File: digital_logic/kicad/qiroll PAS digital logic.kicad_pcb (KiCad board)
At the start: 2 copper layers, 53.3 x 45.7 mm, 43 parts, among them J1 led_sw1, J2 mode_thr_batt, J3 pas_sense, J4 brk_sense, J5 jumper, U1 14538, U2 4023, U3 4027, U4 14538, U5 L7805, U6 4081, U7 4047, U8 74VHC1G32

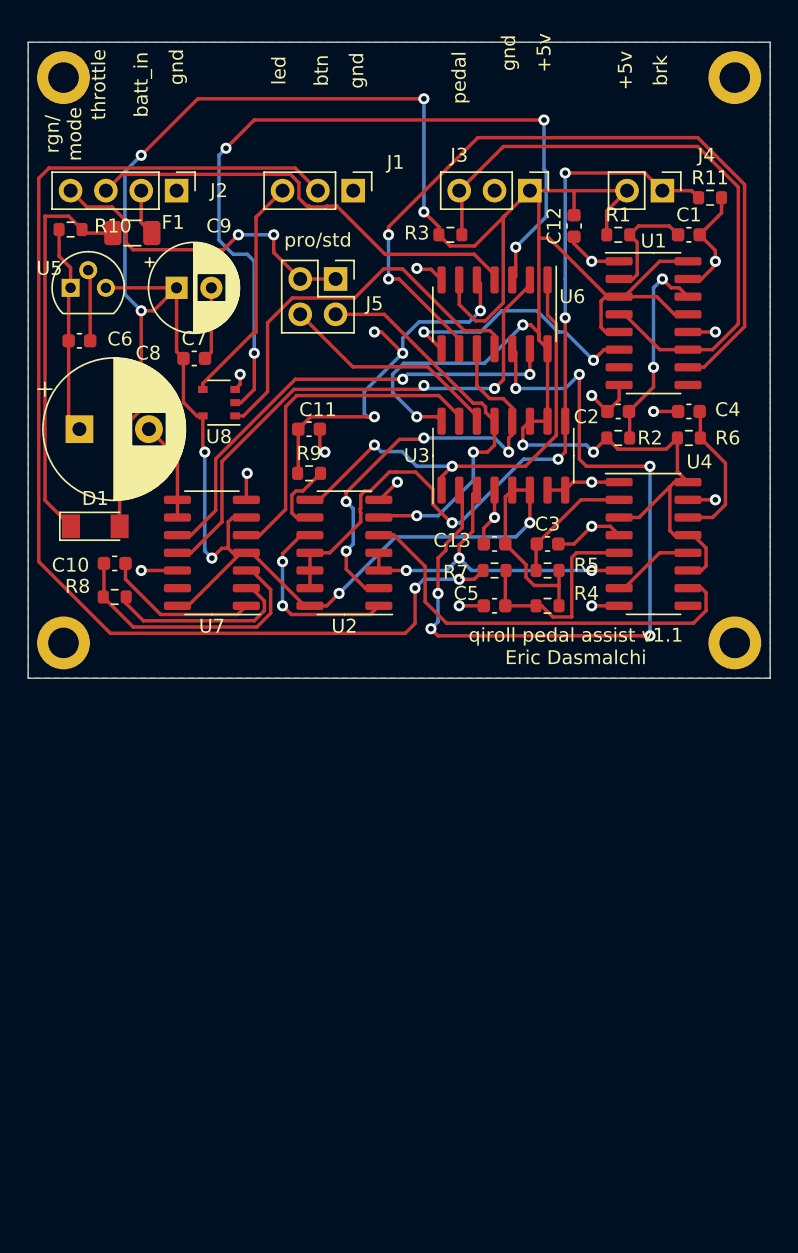
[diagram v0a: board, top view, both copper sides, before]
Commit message: trial component placement
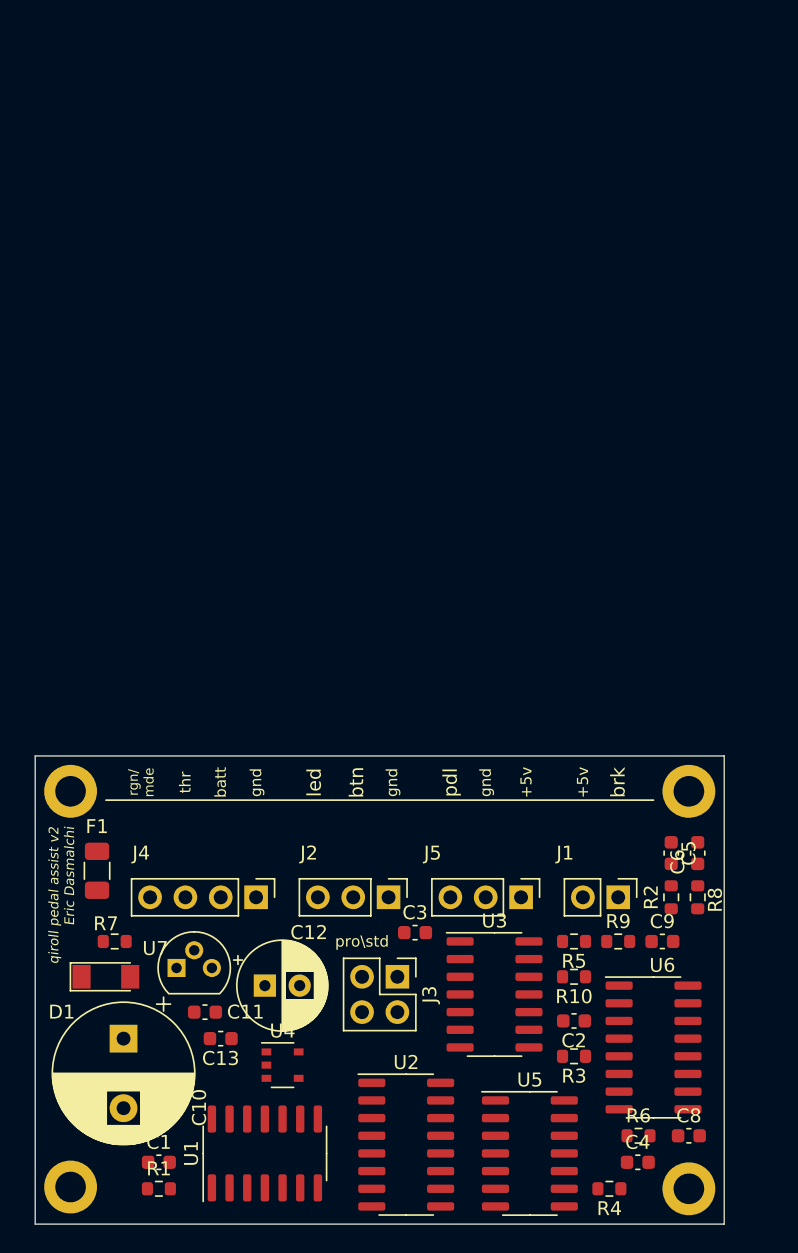
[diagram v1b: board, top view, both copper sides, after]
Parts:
- removed the C11 at (131.4, 70.5)
- removed the C12 at (150.5, 55.9)
- removed C7: .1u, Capacitor_SMD:C_0603_1608Metric
- removed the J1 at (134.6, 53.3)
- removed the J5 at (133.3, 59.7)
- removed R11: 10k, Resistor_SMD:R_0603_1608Metric
- removed the U7 at (124.5, 79.4)
- removed U8: 74VHC1G32, Package_SO:TSOP-5_1.65x3.05mm_P0.95mm
- added C6: .22u, Capacitor_SMD:C_0603_1608Metric, F.Cu at (159.4, 101.0)
- added C9: 4.7u, Capacitor_SMD:C_0603_1608Metric, F.Cu at (156.8, 107.3)
- added J2: led_sw1, Connector_PinHeader_2.54mm:PinHeader_1x03_P2.54mm_Vertical, F.Cu at (137.2, 104.1)
- added J3: jumper, Connector_PinHeader_2.54mm:PinHeader_2x02_P2.54mm_Vertical, F.Cu at (137.8, 109.9)
- added U5: 4023, Package_SO:SOIC-14_3.9x8.7mm_P1.27mm, F.Cu at (147.3, 122.6)
- C10: value 0.47u -> 150u; footprint Capacitor_SMD:C_0603_1608Metric -> Capacitor_THT:CP_Radial_D10.0mm_P5.00mm
- C11: renamed from C6; value 0.47u -> .22u
- C2: value 1u -> .22u
- C3: value 0.47u -> .1u
- C4, C5: value 1u -> .1u
- C8: value 150u -> 1u; footprint Capacitor_THT:CP_Radial_D10.0mm_P5.00mm -> Capacitor_SMD:C_0603_1608Metric
- D1: value Reverse Protect Diode -> LL4150GS18
- F1: value PTC -> 0ZCJ0012FF2E
- R10: value 1.6k -> 73k
- R2: value 200k -> 73k
- R3: value 10k -> 200k
- R4: value 100k -> 392k
- R5: value 100k -> 73k
- R7: value 10k -> 1.6k
- R8: value 100k -> 200k
- R9: value 392K -> 200k
- U1: value 14538 -> CD4093B; footprint Package_SO:SOIC-16_3.9x9.9mm_P1.27mm -> Package_SO:SOIC-14_3.9x8.7mm_P1.27mm
- U2: value 4023 -> 4027; footprint Package_SO:SOIC-14_3.9x8.7mm_P1.27mm -> Package_SO:SOIC-16_3.9x9.9mm_P1.27mm
- U3: value 4027 -> CD4093B; footprint Package_SO:SOIC-16_3.9x9.9mm_P1.27mm -> Package_SO:SOIC-14_3.9x8.7mm_P1.27mm
- U4: value 14538 -> 74VHC1G32; footprint Package_SO:SOIC-16_3.9x9.9mm_P1.27mm -> Package_SO:TSOP-5_1.65x3.05mm_P0.95mm
- U6: value 4081 -> 14538; footprint Package_SO:SOIC-14_3.9x8.7mm_P1.27mm -> Package_SO:SOIC-16_3.9x9.9mm_P1.27mm
- U7: renamed from U5; value L7805 -> 78L05
- moved H1 80.0 mm to (158.8, 125.1)
- moved H2 79.8 mm to (114.3, 125.0)
- moved C1 76.8 mm to (120.7, 123.2)
- moved R1 76.1 mm to (120.7, 125.1)
- moved C8 67.1 mm to (158.8, 121.3)
- moved U1 65.9 mm to (128.3, 122.6), turned to 90 degrees
- moved R10 64.8 mm to (150.5, 109.9), turned to 180 degrees
- moved R3 59.7 mm to (150.5, 115.6), turned to 180 degrees
- moved C4 54.1 mm to (155.1, 123.2), turned to 0 degrees
- moved U6 53.9 mm to (156.2, 114.9), turned to 0 degrees
- moved J4 51.1 mm to (127.6, 104.1)
- moved J1 50.9 mm to (153.7, 104.1)
- moved J5 50.8 mm to (146.7, 104.1)
- moved C12 50.6 mm to (128.3, 110.5)
- moved R6 50.3 mm to (155.1, 121.3)
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- renumbered C9 to C12, J4 to J1, J2 to J4, J3 to J5
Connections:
- C10 pad 2: Net-(C10-Pad2) -> GND
- C11 pad 1: Net-(C6-Pad1) -> Net-(C10-Pad1)
- C13 pad 1: GND -> VCC
- C13 pad 2: VCC -> GND
- C2 pad 1: Net-(C2-Pad1) -> VCC
- C2 pad 2: GND -> Net-(C2-Pad2)
- C3 pad 1: Net-(C3-Pad1) -> GND
- C3 pad 2: GND -> Net-(C3-Pad2)
- C4 pad 1: Net-(C4-Pad1) -> VCC
- C5 pad 1: GND -> Net-(C5-Pad1)
- C5 pad 2: Net-(C5-Pad2) -> GND
- C8 pad 1: Net-(C6-Pad1) -> Net-(C8-Pad1)
- J1 pad 1: BRK -> Net-(J1-Pad1)
- J4 pad 3: Net-(J2-Pad3) -> Net-(J4-Pad3)
- J5 pad 3: Net-(J3-Pad3) -> Net-(J5-Pad3)
- R1 pad 1: VCC -> Net-(R1-Pad1)
- R10 pad 1: Net-(C6-Pad1) -> Net-(R10-Pad1)
- R10 pad 2: Net-(D1-Pad1) -> Net-(C9-Pad1)
- R2 pad 1: VCC -> Net-(J1-Pad1)
- R2 pad 2: Net-(C2-Pad1) -> GND
- R3 pad 2: Net-(J3-Pad3) -> Net-(C2-Pad2)
- R4 pad 1: VCC -> Net-(C3-Pad2)
- R4 pad 2: Net-(C5-Pad2) -> Net-(R4-Pad2)
- R5 pad 2: Net-(C3-Pad1) -> Net-(J5-Pad3)
- R6 pad 2: Net-(C4-Pad1) -> Net-(C8-Pad1)
- R7 pad 1: Net-(J1-Pad2) -> Net-(C10-Pad1)
- R7 pad 2: Net-(C5-Pad2) -> Net-(D1-Pad1)
- R8 pad 1: Net-(C10-Pad2) -> VCC
- R8 pad 2: Net-(R8-Pad2) -> Net-(C5-Pad1)
- R9 pad 1: Net-(C11-Pad2) -> VCC
- R9 pad 2: Net-(R9-Pad2) -> Net-(C9-Pad1)
- U1 pad 1: GND -> Net-(C1-Pad1)
- U1 pad 11: Net-(J3-Pad3) -> Net-(U1-Pad11)
- U1 pad 12: GND -> Net-(U1-Pad12)
- U1 pad 13: VCC -> Net-(R1-Pad1)
- U1 pad 14: Net-(C2-Pad1) -> VCC
- U1 pad 2: Net-(C1-Pad1) -> Net-(U1-Pad2)
- U1 pad 3: VCC -> Net-(R1-Pad1)
- U1 pad 4: Net-(J3-Pad3) -> Net-(U1-Pad4)
- U1 pad 5: VCC -> Net-(R1-Pad1)
- U1 pad 6: Net-(U1-Pad6) -> Net-(R1-Pad1)
- U1 pad 7: Net-(U1-Pad7) -> GND
- U1 pad 8: GND -> Net-(U1-Pad4)
- U2 pad 1: Net-(U2-Pad1) -> Net-(U1-Pad12)
- U2 pad 10: Net-(U2-Pad1) -> VCC
- U2 pad 11: BRK -> VCC
- U2 pad 12: BRK -> Net-(U2-Pad12)
- U2 pad 13: BRK -> Net-(J3-Pad2)
- U2 pad 14: VCC -> Net-(J3-Pad4)
- U2 pad 2: PEDAL -> Net-(U1-Pad9)
- U2 pad 4: Net-(U2-Pad3) -> GND
- U2 pad 5: Net-(U2-Pad5) -> VCC
- U2 pad 6: Net-(J5-Pad2) -> VCC
- U2 pad 8: PAS_ON -> GND
- U2 pad 9: Net-(R9-Pad2) -> Net-(J1-Pad1)
- U3 pad 1: PAS_ON -> Net-(C3-Pad2)
- U3 pad 10: VCC -> Net-(U2-Pad3)
- U3 pad 11: VCC -> Net-(U2-Pad12)
- U3 pad 12: PEDAL -> Net-(C9-Pad1)
- U3 pad 13: Net-(J5-Pad2) -> VCC
- U3 pad 14: Net-(J5-Pad4) -> VCC
- U3 pad 2: PAS_OFF -> Net-(C3-Pad2)
- U3 pad 3: Net-(U2-Pad3) -> Net-(U3-Pad3)
- U3 pad 4: GND -> Net-(J4-Pad3)
- U3 pad 5: VCC -> Net-(U3-Pad3)
- U3 pad 6: VCC -> Net-(U3-Pad3)
- U3 pad 8: GND -> Net-(C2-Pad2)
- U3 pad 9: BRK -> VCC
- U4 pad 1: GND -> Net-(U1-Pad10)
- U4 pad 2: Net-(C3-Pad1) -> Net-(U1-Pad11)
- U4 pad 3: VCC -> GND
- U4 pad 4: GND -> Net-(J2-Pad3)
- U4 pad 5: Net-(C5-Pad2) -> VCC
- U6 pad 1: PAS_ON -> GND
- U6 pad 10: PEDAL -> GND
- U6 pad 11: RGN_FLSH_2 -> Net-(U2-Pad3)
- U6 pad 12: PAS_OFF -> GND
- U6 pad 13: Net-(U6-Pad13) -> VCC
- U6 pad 14: VCC -> Net-(C8-Pad1)
- U6 pad 2: RGN_FLSH -> Net-(C5-Pad1)
- U6 pad 3: Net-(U6-Pad3) -> VCC
- U6 pad 4: Net-(J2-Pad3) -> Net-(J5-Pad3)
- U6 pad 5: Net-(C11-Pad2) -> VCC
- U6 pad 6: VCC -> Net-(R10-Pad1)
- U6 pad 7: GND -> Net-(U6-Pad7)
- U6 pad 8: Net-(U1-Pad6) -> GND
- U6 pad 9: Net-(U1-Pad10) -> Net-(U6-Pad9)
- U7 pad 1: Net-(C6-Pad1) -> Net-(C10-Pad1)
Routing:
- net VCC: track 270.2 -> 0.00 mm, vias 12 -> 0
- net Net-(J1-Pad2): track 86.0 -> 0.00 mm, vias 2 -> 0
- net GND: track 70.0 -> 0.00 mm, vias 17 -> 0
- net BRK: track 60.5 -> 0.00 mm, vias 4 -> 0
- net PAS_OFF: track 58.5 -> 0.00 mm, vias 6 -> 0
- net Net-(U6-Pad3): track 57.2 -> 0.00 mm, vias 4 -> 0
- net Net-(U1-Pad10): track 56.5 -> 0.00 mm, vias 2 -> 0
- net Net-(J3-Pad3): track 46.1 -> 0.00 mm
- net RGN_FLSH: track 39.6 -> 0.00 mm, vias 2 -> 0
- net Net-(U6-Pad13): track 35.0 -> 0.00 mm, vias 2 -> 0
- net PAS_ON: track 34.4 -> 0.00 mm, vias 2 -> 0
- net PEDAL: track 32.8 -> 0.00 mm, vias 4 -> 0
- net Net-(J2-Pad3): track 32.5 -> 0.00 mm
- net Net-(U2-Pad5): track 31.7 -> 0.00 mm
- net RGN_FLSH_2: track 28.9 -> 0.00 mm
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- removed copper zone on B.Cu, net GND
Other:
- board size 53.3 x 45.7 mm -> 49.5 x 33.7 mm
- net class Default: clearance 0.2 -> 0.15; trace_width 0.25 -> 0.15; via_dia 0.8 -> 0.65; via_drill 0.4 -> 0.35
- rule trace_clearance: 0.2 -> 0.15
- rule trace_min: 0.2 -> 0.15
- board text added: "batt"
- board text added: "pdl"
- board text added: "pro\std"
- board text added: "qiroll pedal assist v2 Eric Dasmalchi"
- board text added: "rgn/ mde"
- board text added: "thr"
- board text removed: "batt_in"
- board text removed: "pedal"
- board text removed: "pro/std"
- board text removed: "qiroll pedal assist v1.1 Eric Dasmalchi"
- board text removed: "rgn/ mode"
- board text removed: "throttle"
